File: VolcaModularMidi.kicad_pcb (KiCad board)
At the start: 2 copper layers, 30 x 18.2 mm, 6 parts, among them J1 Conn_01x04_Male, J2 MIDI_IN, U1 6N139

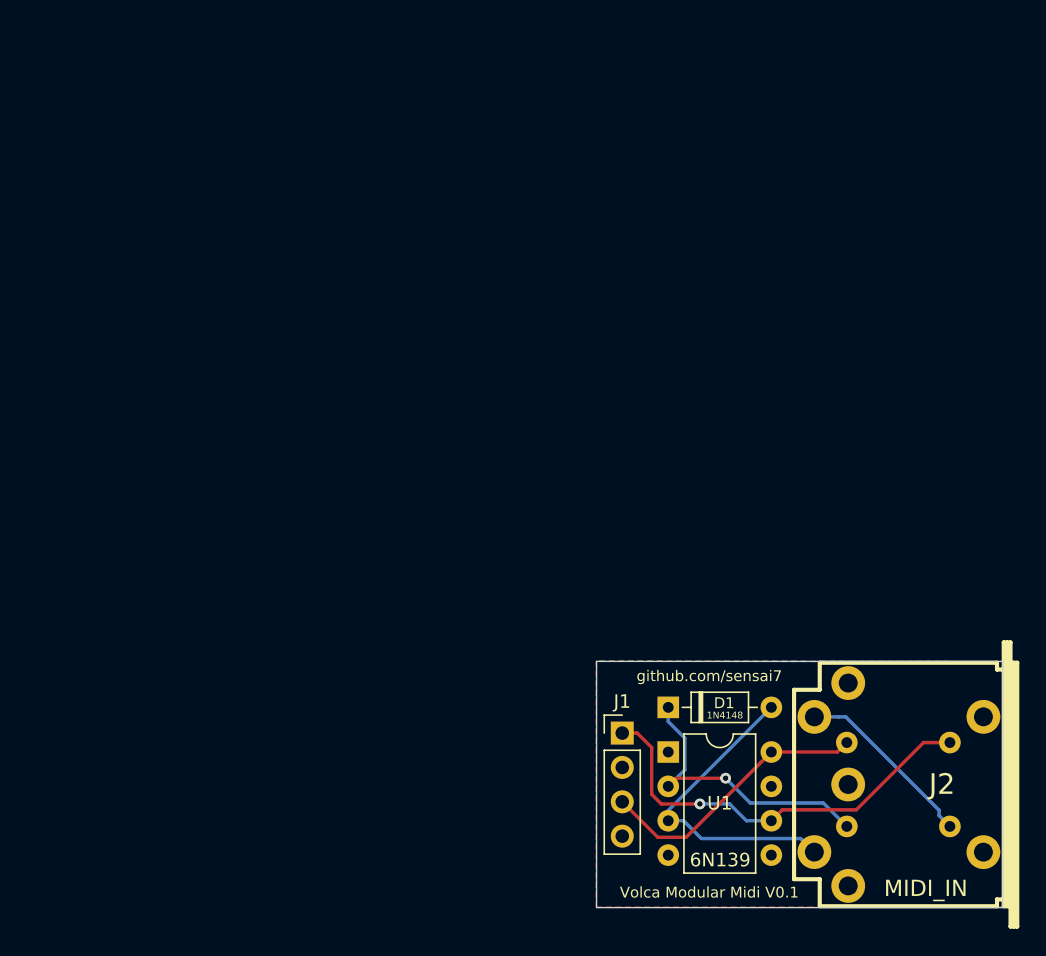
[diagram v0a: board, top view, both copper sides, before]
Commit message: Finished routing and laying out pcb
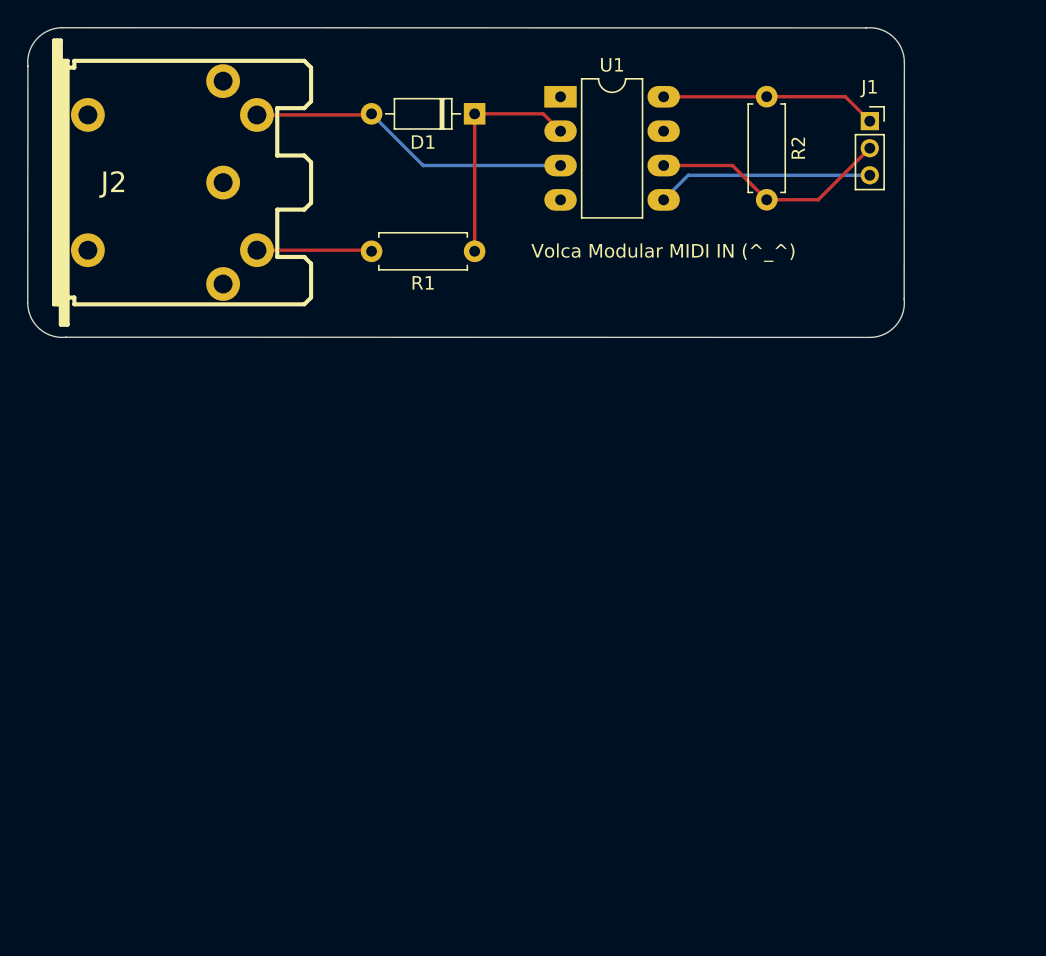
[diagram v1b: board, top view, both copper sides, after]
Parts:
- J1: value Conn_01x04_Male -> Conn_01x03_Female; footprint Connector_PinHeader_2.54mm:PinHeader_1x04_P2.54mm_Vertical -> Connector_PinSocket_2.00mm:PinSocket_1x03_P2.00mm_Vertical
- J2: value MIDI_IN -> (none); footprint SensaiLib:din-5 -> eurocad:MIDI_DIN5
- R1, R2: moved to F.Cu
- U1: value 6N139 -> 6N137; footprint Package_DIP:DIP-8_W7.62mm -> Package_DIP:DIP-8_W7.62mm_LongPads
- moved J2 68.6 mm to (86.4, 71.1), turned to -90 degrees
- moved R1 50.6 mm to (108.0, 76.2), turned to 180 degrees
- moved U1 49.1 mm to (114.3, 64.8)
- moved J1 48.8 mm to (137.2, 66.6)
- moved R2 48.1 mm to (129.5, 64.8), turned to -90 degrees
- moved D1 46.1 mm to (108.0, 66.0), turned to 180 degrees
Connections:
- J1 pad 1: RX -> VCC
- J1 pad 2: TX -> RX
- J1 pad 3: VCC -> GND
- J2 pad 1: Net-(J2-Pad1) -> unconnected-(J2-Pad1)
- J2 pad 2: Net-(J2-Pad2) -> unconnected-(J2-Pad2)
- J2 pad 3: Net-(J2-Pad3) -> unconnected-(J2-Pad3)
- U1 pad 1: Net-(U1-Pad1) -> unconnected-(U1-Pad1)
- U1 pad 4: Net-(U1-Pad4) -> unconnected-(U1-Pad4)
- U1 pad 7: Net-(U1-Pad7) -> unconnected-(U1-Pad7)
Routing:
- net GND: track 0.00 -> 16.0 mm
- net RX: track 31.3 -> 17.9 mm, vias 1 -> 0
- net Net-(J2-Pad4): track 13.6 -> 8.51 mm
- net Net-(D1-Pad1): track 21.8 -> 17.0 mm, vias 1 -> 0
- net VCC: track 20.6 -> 16.0 mm
- net Net-(D1-Pad2): track 23.3 -> 24.1 mm
- removed copper zone on B.Cu, net GND
- removed copper zone on F.Cu, net GND
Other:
- board size 30 x 18.2 mm -> 64.8 x 22.9 mm
- net class Default removed
- rule pad_to_mask_clearance: 0.051 -> 0
- board text added: "Volca Modular MIDI IN (^_^)"
- board text removed: "+"
- board text removed: "-"
- board text removed: "R"
- board text removed: "T"
- board text removed: "Volca Modular Midi V0.1"
- board text removed: "github.com/sensai7"
